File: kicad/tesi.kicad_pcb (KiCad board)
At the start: 4 copper layers, 100 x 100 mm, 34 parts, among them J3 Conn_01x04_Pin, SW1 POWER, U1 MAX4466, U2 BNO055

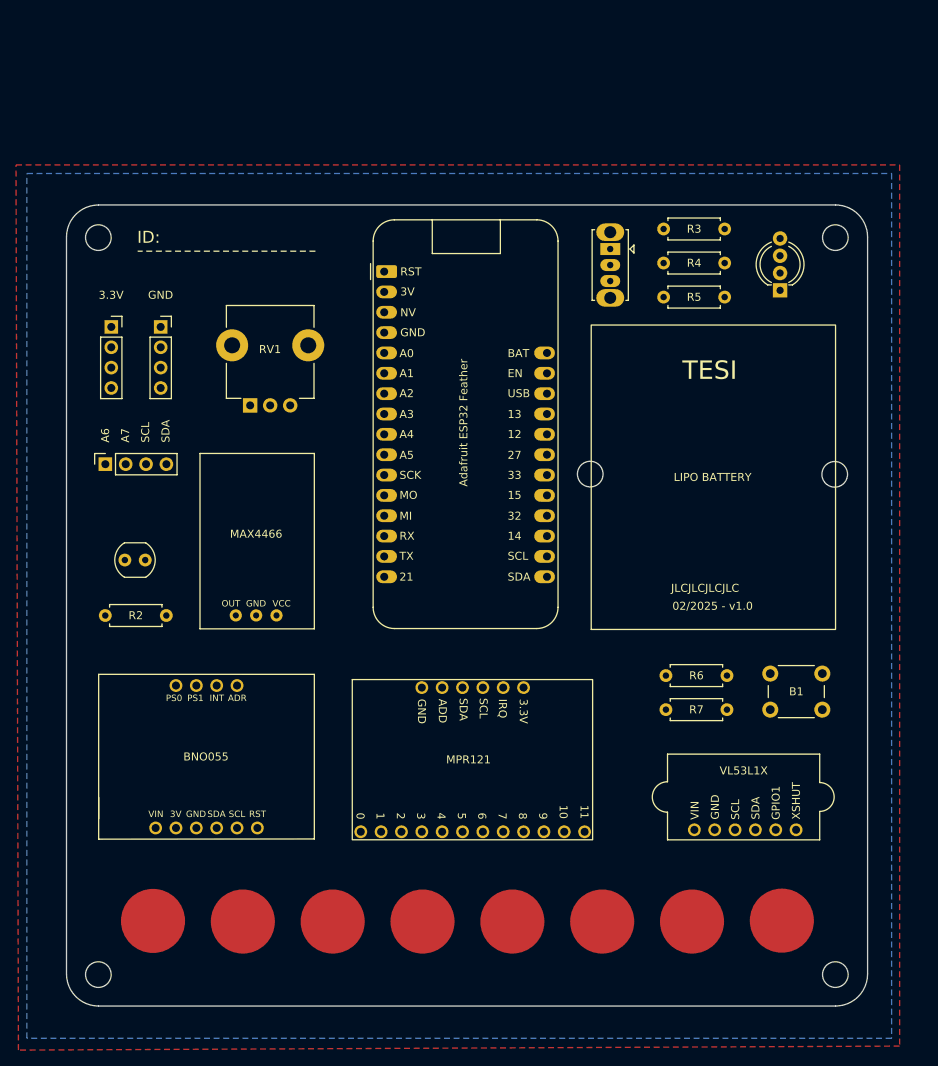
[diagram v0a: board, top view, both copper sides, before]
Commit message: update pcb
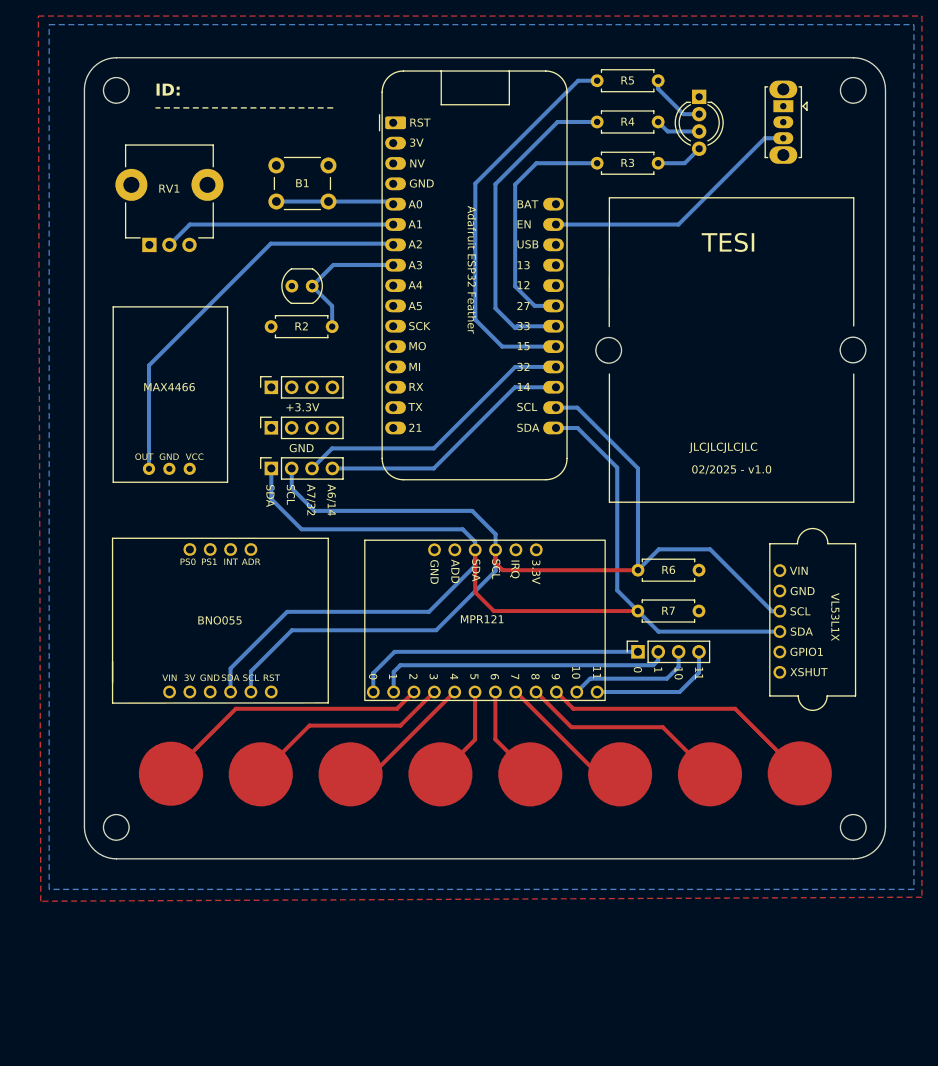
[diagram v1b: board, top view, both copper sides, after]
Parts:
- removed BT1: LIPO BATTERY, tesi:Lipo Battery 500 mAh - 38x30.5mm
- added J4: Conn_01x04_Pin, Connector_PinSocket_2.54mm:PinSocket_1x04_P2.54mm_Vertical, F.Cu at (119.8, 107.3)
- added REF**: Perfboard_10x10, tesi:Perfboard_10x10, F.Cu at (48.6, 31.1)
- A2: value Adafruit ESP32 Feather -> Adafruit Feather HUZZAH32; footprint tesi:Adafruit HUZZAH32 Feather Board - WithoutMountingHoles -> tesi:Adafruit ESP32 Feather
- moved B1 96.2 mm to (74.6, 46.6), turned to 0 degrees
- moved R1 41.4 mm to (79.1, 61.6), turned to 180 degrees
- moved R2 38.4 mm to (74.0, 66.7), turned to 0 degrees
- moved R5 28.3 mm to (122.3, 36.0)
- moved SW1 28.0 mm to (137.9, 39.2)
- moved D1 26.2 mm to (127.4, 38.0), turned to -90 degrees
- moved U4 23.8 mm to (141.5, 103.3), turned to -90 degrees
- moved RV1 23.7 mm to (58.8, 56.5)
- moved +3.3V 21.4 mm to (74.0, 74.3), turned to 90 degrees
- moved U1 21.3 mm to (61.3, 74.3)
- moved J3 20.7 mm to (74.0, 84.4)
- moved R4 19.5 mm to (122.3, 41.1)
- moved GND 18.7 mm to (74.0, 79.3), turned to 90 degrees
- moved A2 18.6 mm to (89.2, 41.2)
- moved H3 18.5 mm to (54.6, 37.2)
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- renumbered 3.3V to +3.3V, MPR121 to U3, VL53L1X to U4
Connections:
- A2 pad 5: unconnected-(A2-DAC2/A0-Pad5) -> Net-(A2-DAC2/A0)
- A2 pad 9: Net-(A2-IO36/A4) -> unconnected-(A2-IO36/A4-Pad9)
- B1 pad 2: Net-(A2-DAC1/A1) -> Net-(A2-DAC2/A0)
- J3 pad 1: Net-(A2-A6/IO14) -> SDA
- J3 pad 2: Net-(A2-A7/IO32) -> SCL
- J3 pad 3: SCL -> Net-(A2-A7/IO32)
- J3 pad 4: SDA -> Net-(A2-A6/IO14)
- R1 pad 1: Net-(A2-IO36/A4) -> Net-(A2-I39/A3)
- R2 pad 2: Net-(A2-IO36/A4) -> Net-(A2-I39/A3)
- RV1 pad 2: Net-(A2-I34/A2) -> Net-(A2-DAC1/A1)
- TP1 pad 1: Net-(U3-ELE1) -> Net-(U3-ELE2)
- TP2 pad 1: Net-(U3-ELE2) -> Net-(U3-ELE3)
- TP3 pad 1: Net-(U3-ELE3) -> Net-(U3-LED0/ELE4)
- TP4 pad 1: Net-(U3-LED0/ELE4) -> Net-(U3-LED1/ELE5)
- TP5 pad 1: Net-(U3-LED1/ELE5) -> Net-(U3-LED2/ELE6)
- TP6 pad 1: Net-(U3-LED2/ELE6) -> Net-(U3-LED3/ELE7)
- TP7 pad 1: Net-(U3-LED3/ELE7) -> Net-(U3-LED4/ELE8)
- TP8 pad 1: Net-(U3-LED4/ELE8) -> Net-(U3-LED5/ELE9)
- U1 pad 3: Net-(A2-I39/A3) -> Net-(A2-I34/A2)
- U2 pad 4: +3.3V -> unconnected-(U2-3V-Pad4)
- U3 pad 17: unconnected-(U3-LED5/ELE9-Pad17) -> Net-(U3-LED5/ELE9)
- U3 pad 18: unconnected-(U3-LED6/ELE10-Pad18) -> Net-(J4-Pin_3)
- U3 pad 19: unconnected-(U3-LED7/ELE11-Pad19) -> Net-(J4-Pin_4)
- U3 pad 2: SCL -> unconnected-(U3-ADDR-Pad2)
- U3 pad 4: unconnected-(U3-ADDR-Pad4) -> SCL
- U3 pad 5: +3.3V -> unconnected-(U3-IRQ-Pad5)
- U3 pad 6: unconnected-(U3-GND-Pad6) -> +3.3V
- U3 pad 8: unconnected-(U3-ELE0-Pad8) -> Net-(J4-Pin_1)
- U3 pad 9: Net-(U3-ELE1) -> Net-(J4-Pin_2)
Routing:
- net SDA: track 0.00 -> 147.3 mm
- net SCL: track 0.00 -> 141.1 mm
- net Net-(A2-I34/A2): track 0.00 -> 49.7 mm
- net Net-(A2-A8/IO15): track 0.00 -> 49.0 mm
- net Net-(A2-A9/IO33): track 0.00 -> 40.1 mm
- net Net-(J4-Pin_2): track 0.00 -> 37.2 mm
- net Net-(J4-Pin_1): track 0.00 -> 36.5 mm
- net Net-(A2-A7/IO32): track 0.00 -> 35.7 mm
- net Net-(U3-LED5/ELE9): track 0.00 -> 34.6 mm
- net Net-(U3-ELE2): track 0.00 -> 34.6 mm
- net Net-(A2-EN): track 0.00 -> 32.8 mm
- net Net-(A2-A6/IO14): track 0.00 -> 32.1 mm
- net Net-(A2-A10/IO27): track 0.00 -> 30.1 mm
- net Net-(A2-DAC1/A1): track 0.00 -> 29.0 mm
- net Net-(U3-LED4/ELE8): track 0.00 -> 26.0 mm
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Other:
- copper layers 4 -> 2
- board text added: "0"
- board text added: "1"
- board text added: "10"
- board text added: "11"
- board text added: "A6/14"
- board text added: "A7/32"
- board text added: "Adafruit ESP32 Feather"
- board text added: "MPR121"
- board text added: "VL53L1X"
- board text removed: "A6"
- board text removed: "A7"
